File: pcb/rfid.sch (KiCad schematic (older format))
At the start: 54 parts, among them IC1 EM4095, IC2 ATTINY13A-SS, J1 USB

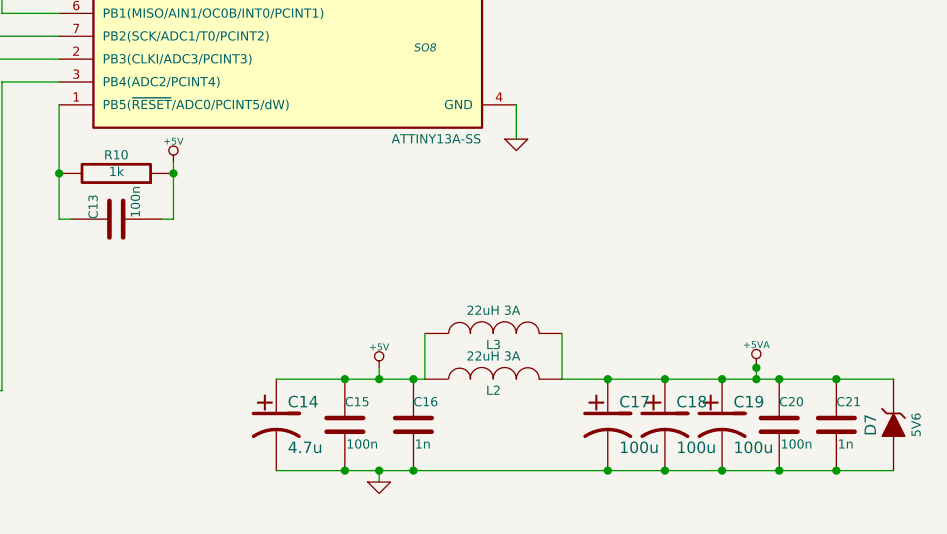
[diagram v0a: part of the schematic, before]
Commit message: starting new pcb routing
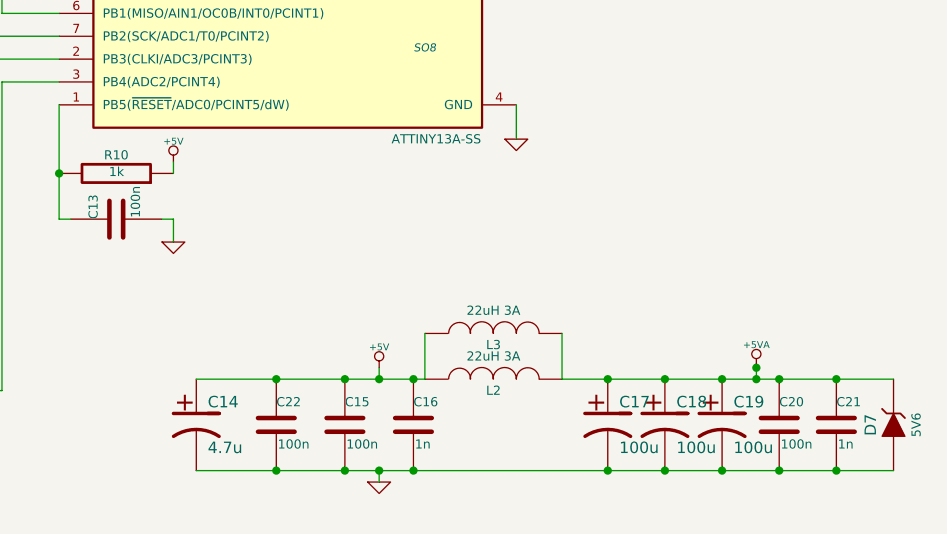
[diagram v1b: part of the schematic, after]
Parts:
- added C22: 100n, ~, symbol C
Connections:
- net +5V: now also C22.1; no longer C13.2
- net GND: now also C13.2, C22.2
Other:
- moved on the sheet: C14
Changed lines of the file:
@@
 Sheet 1 1
 Title ""
-Date "20 sep 2014"
+Date "26 sep 2014"
 Rev ""
 Comp ""
@@
 L CP1 C14
 U 1 1 54130039
-P 7900 6150
-F 0 "C14" H 7950 6250 50  0000 L CNN
-F 1 "4.7u" H 7950 6050 50  0000 L CNN
-F 2 "~" H 7900 6150 60  0000 C CNN
-F 3 "~" H 7900 6150 60  0000 C CNN
-	1    7900 6150
+P 7550 6150
+F 0 "C14" H 7600 6250 50  0000 L CNN
+F 1 "4.7u" H 7600 6050 50  0000 L CNN
+F 2 "~" H 7550 6150 60  0000 C CNN
+F 3 "~" H 7550 6150 60  0000 C CNN
+	1    7550 6150
 	1    0    0    -1
 $EndComp
@@
 	5050 2600 5100 2600
 Wire Wire Line
-	7900 5950 8550 5950
-Wire Wire Line
-	7900 6350 10600 6350
+	7550 5950 8550 5950
+Wire Wire Line
+	7550 6350 10600 6350
 Wire Wire Line
 	8350 6400 8350 6350
@@
 	8950 4250 8950 4150
 Wire Wire Line
-	7450 5000 7450 5250
-Wire Wire Line
 	6950 4750 6950 5250
 Wire Wire Line
@@
 Connection ~ 6950 5050
 Wire Wire Line
-	7450 5250 7400 5250
-Connection ~ 7450 5050
-Wire Wire Line
 	8250 1200 6750 1200
 Wire Wire Line
@@
 Wire Wire Line
 	8550 5950 8550 5750
+$Comp
+L GND #PWR025
+U 1 1 54255A0A
+P 7450 5350
+F 0 "#PWR025" H 7450 5350 30  0001 C CNN
+F 1 "GND" H 7450 5280 30  0001 C CNN
+F 2 "" H 7450 5350 60  0001 C CNN
+F 3 "" H 7450 5350 60  0001 C CNN
+	1    7450 5350
+	1    0    0    -1
+$EndComp
+Wire Wire Line
+	7400 5250 7450 5250
+Wire Wire Line
+	7450 5250 7450 5350
+Wire Wire Line
+	7450 5050 7450 5000
+$Comp
+L C C22
+U 1 1 54255D02
+P 7900 6150
+F 0 "C22" H 7900 6250 40  0000 L CNN
+F 1 "100n" H 7906 6065 40  0000 L CNN
+F 2 "~" H 7938 6000 30  0000 C CNN
+F 3 "~" H 7900 6150 60  0000 C CNN
+	1    7900 6150
+	1    0    0    -1
+$EndComp
+Connection ~ 7900 5950
+Connection ~ 7900 6350
 $EndSCHEMATC
